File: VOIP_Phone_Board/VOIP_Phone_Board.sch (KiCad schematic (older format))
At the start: 14 parts, among them J2 Display, J3 KeypadConnector, J4 Hook, J7 Control Buttons, P1 Conn_02x20_Odd_Even

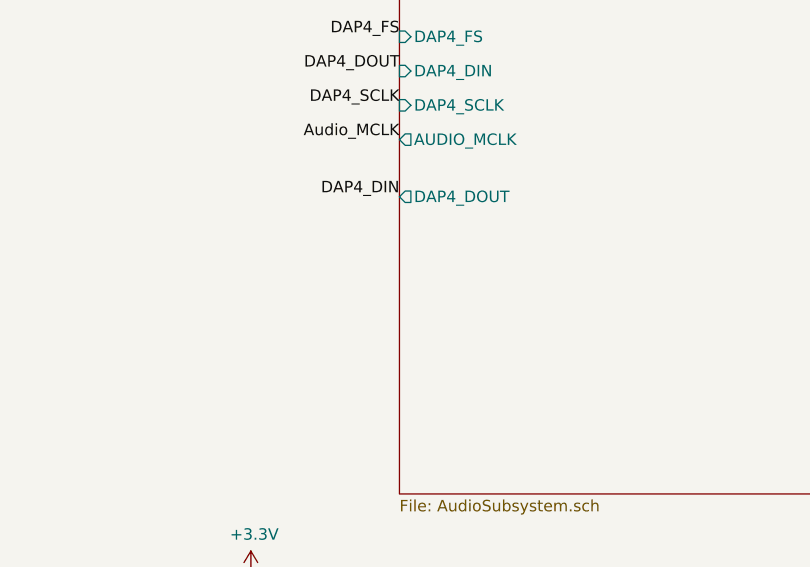
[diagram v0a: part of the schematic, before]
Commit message: MAX98357A Version.
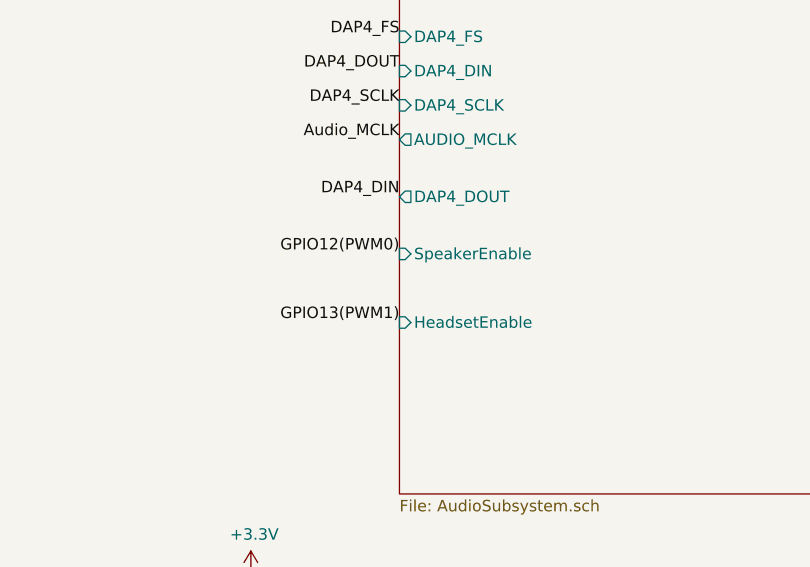
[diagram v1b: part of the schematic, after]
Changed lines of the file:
@@
 F5 "AUDIO_MCLK" O L 6600 2300 50
 F6 "DAP4_DOUT" O L 6600 2550 50
+F7 "SpeakerEnable" I L 6600 2800 50
+F8 "HeadsetEnable" I L 6600 3100 50
 $EndSheet
 Text Label 6600 1850 2    50   ~ 0
@@
 Text Label 5450 5150 2    50   ~ 0
 GPIO8(SPI0_CE_N)
+Text Label 6600 2800 2    50   ~ 0
+GPIO12(PWM0)
+Text Label 6600 3100 2    50   ~ 0
+GPIO13(PWM1)
 $EndSCHEMATC

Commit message: Started with ADAU1361.
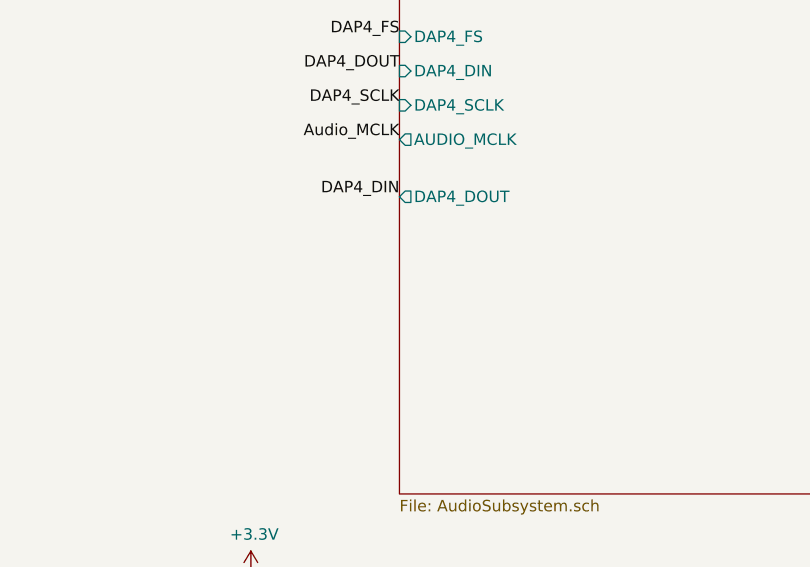
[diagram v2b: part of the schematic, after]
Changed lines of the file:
@@
 F5 "AUDIO_MCLK" O L 6600 2300 50
 F6 "DAP4_DOUT" O L 6600 2550 50
-F7 "SpeakerEnable" I L 6600 2800 50
-F8 "HeadsetEnable" I L 6600 3100 50
 $EndSheet
 Text Label 6600 1850 2    50   ~ 0
@@
 Text Label 5450 5150 2    50   ~ 0
 GPIO8(SPI0_CE_N)
-Text Label 6600 2800 2    50   ~ 0
-GPIO12(PWM0)
-Text Label 6600 3100 2    50   ~ 0
-GPIO13(PWM1)
 $EndSCHEMATC
